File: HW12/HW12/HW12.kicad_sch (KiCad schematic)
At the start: 68 parts, among them J1 Barrel_Jack_MountingPin, Q1 BC337, U1 MC34063AP, U2 LM7805_TO220, U3 NE555P, U4 74HC595, U5 74HC595, U6 74HC595

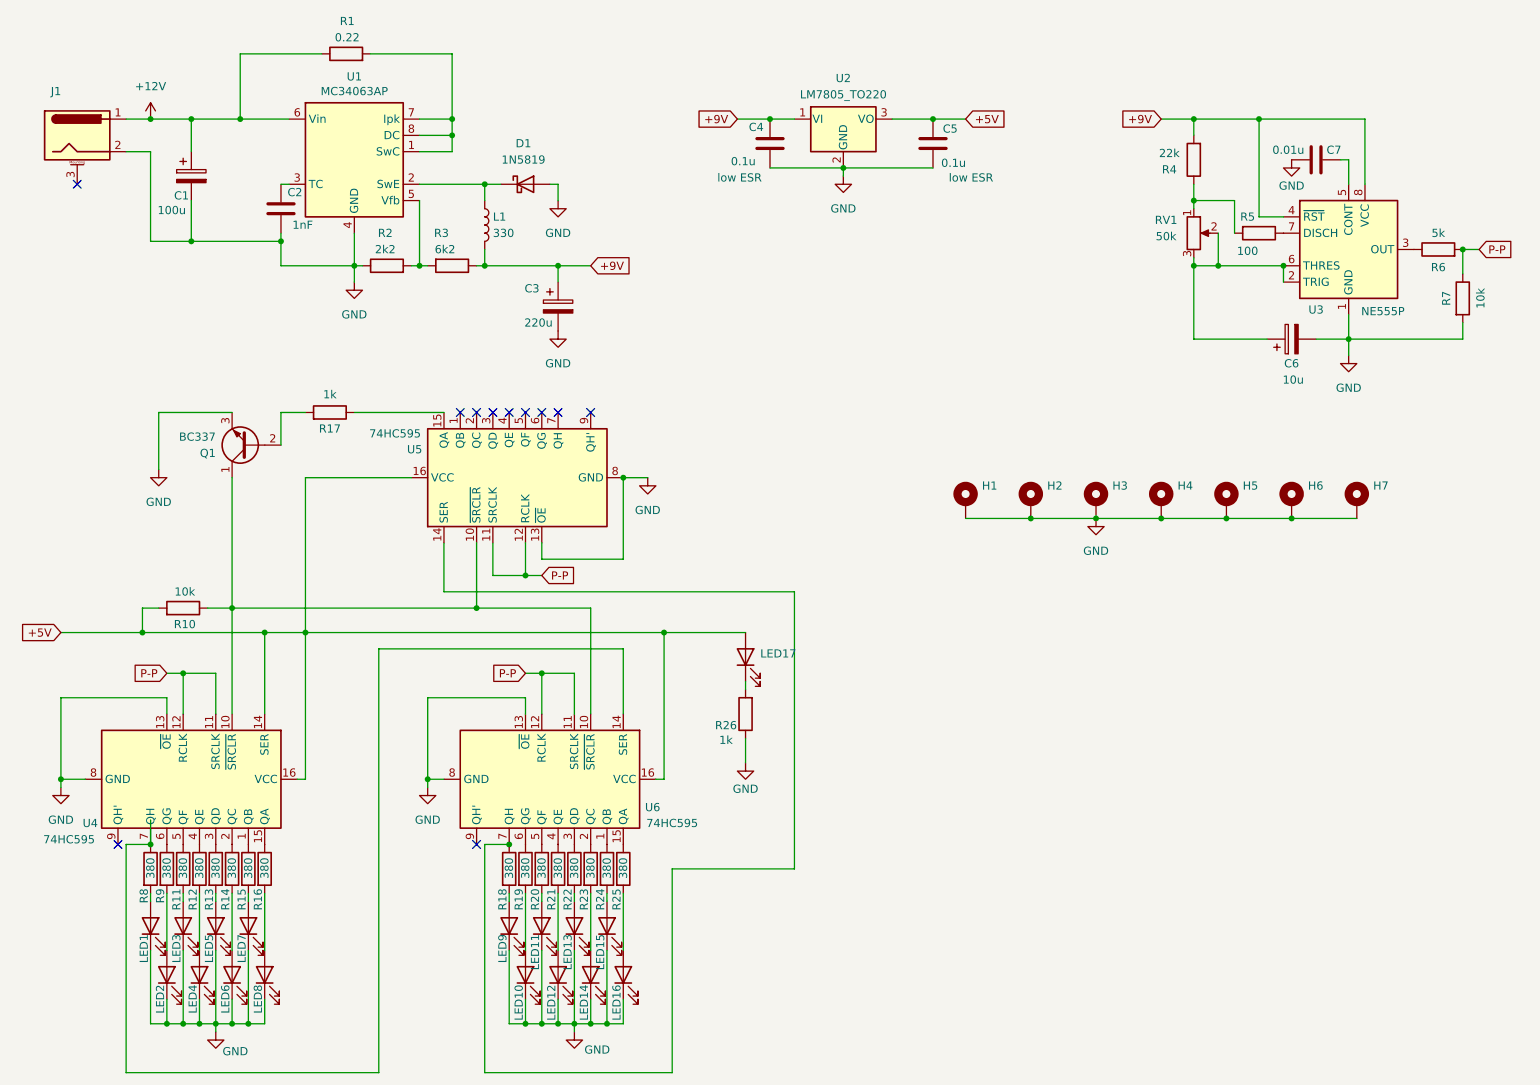
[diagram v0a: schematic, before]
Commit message: hw12 corr
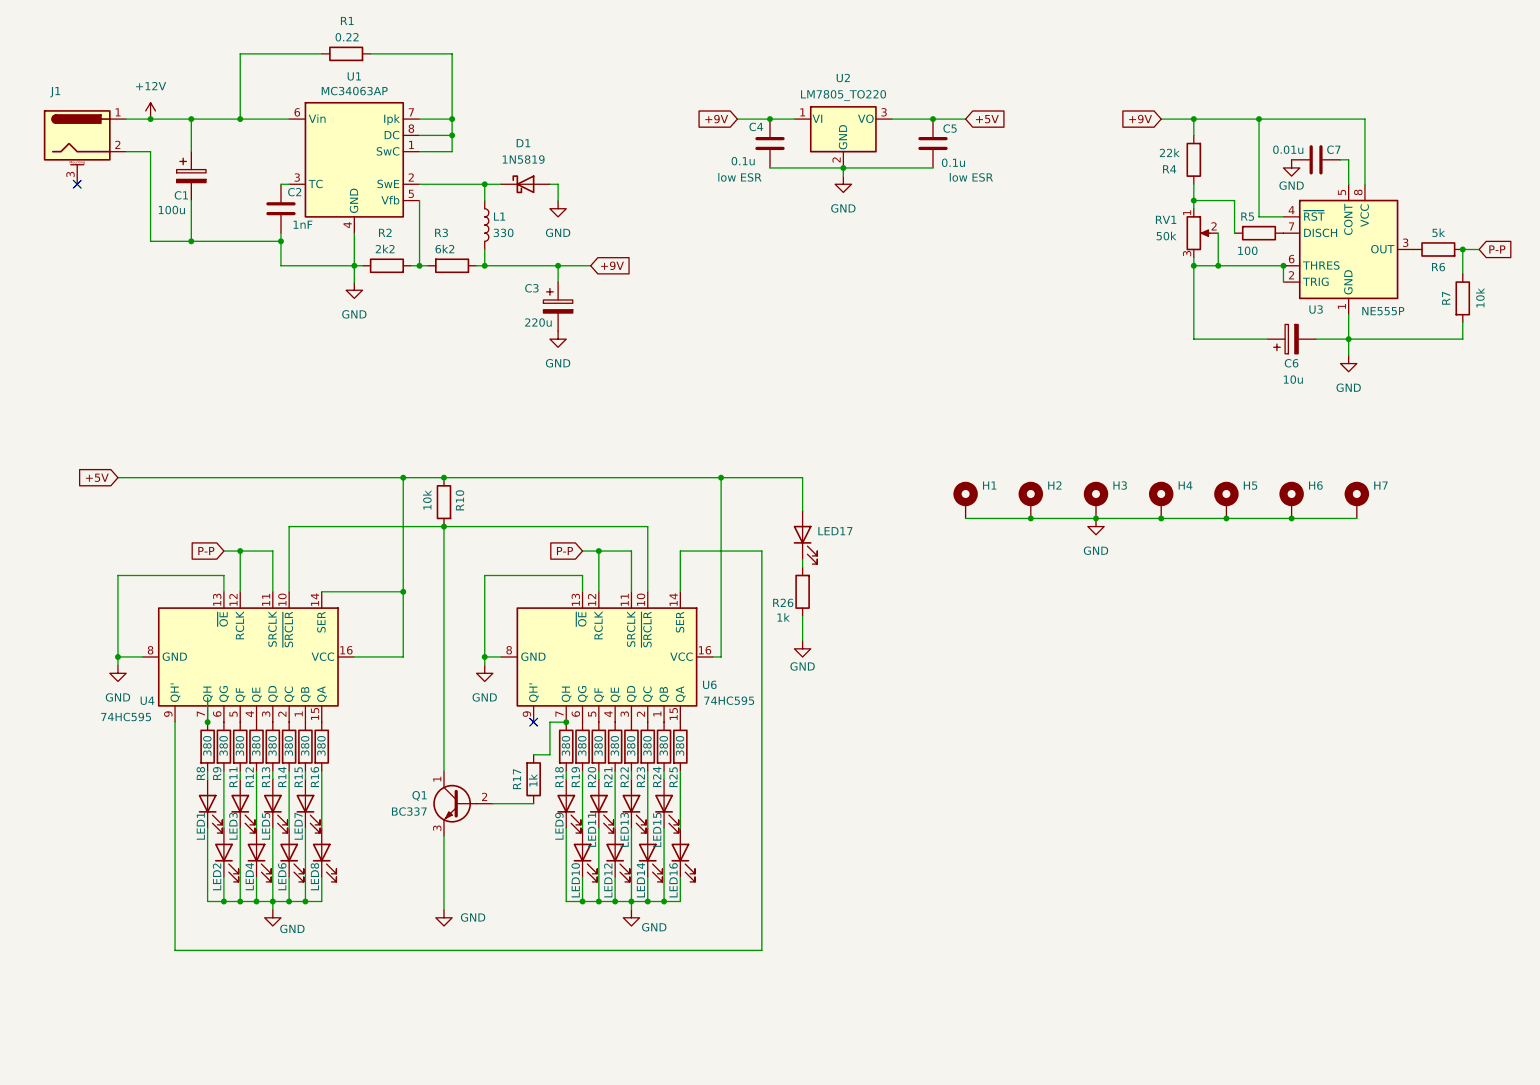
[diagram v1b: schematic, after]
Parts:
- removed U5: 74HC595, Package_DIP:DIP-16_W7.62mm, symbol 74xx:74HC595
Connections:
- net +5V: now also R10.1; no longer R10.2
- net at Q1.1 (C), U4.10 (~{SRCLR}), U6.10 (~{SRCLR}): now also R10.2; no longer R10.1
- net at Q1.2 (B): now also R17.1; no longer R17.2
- net at R8.1, U4.7 (QH): no longer U6.14 (SER)
- net at U4.9 (QH'): now also U6.14 (SER)
- net at R18.1, U6.7 (QH): now also R17.2
- no-connect marks 11 -> 2
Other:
- moved on the sheet: LED1, LED10, LED11, LED12, LED13, LED14, LED15, LED16, LED17, LED2, LED3, LED4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

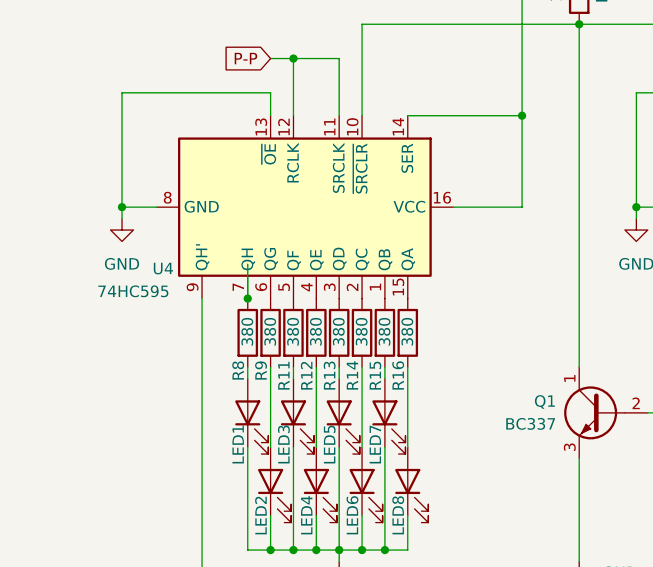
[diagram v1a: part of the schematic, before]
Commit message: HW13 started
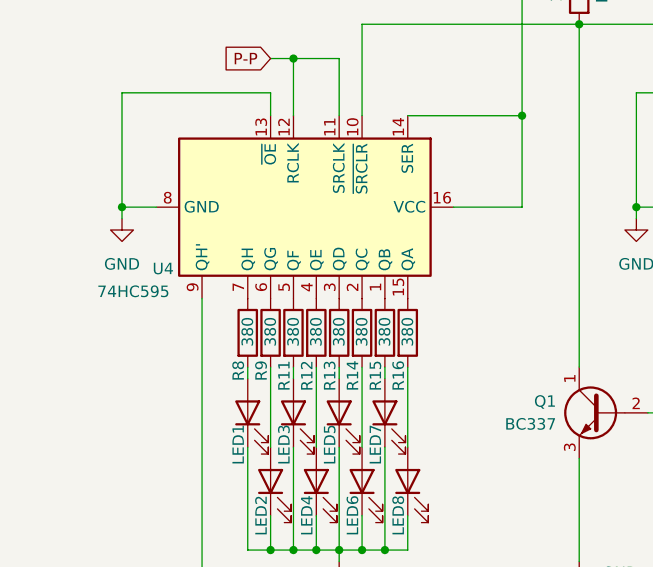
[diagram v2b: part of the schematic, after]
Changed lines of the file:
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@@
-	)
-	(junction
-		(at 60.96 134.62)
-		(diameter 0)
-		(color 0 0 0 0)
 	)
 	(junction
@@
 		)
 		(stroke
-			(width 0)
-			(type default)
-		)
-	)
-	(wire
-		(pts
-			(xy 60.96 130.81) (xy 60.96 134.62)
-		)
-		(stroke
